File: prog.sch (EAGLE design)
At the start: 49 parts, among them IC2 LD398533RM, IC3 74AHCT1G04DBV, Q1 220mA/50V/3.5Ω, T1 SS8050-G, T2 SS8050-G, U1 SN74AHC125PWR, U2 FT2232HL-REEL

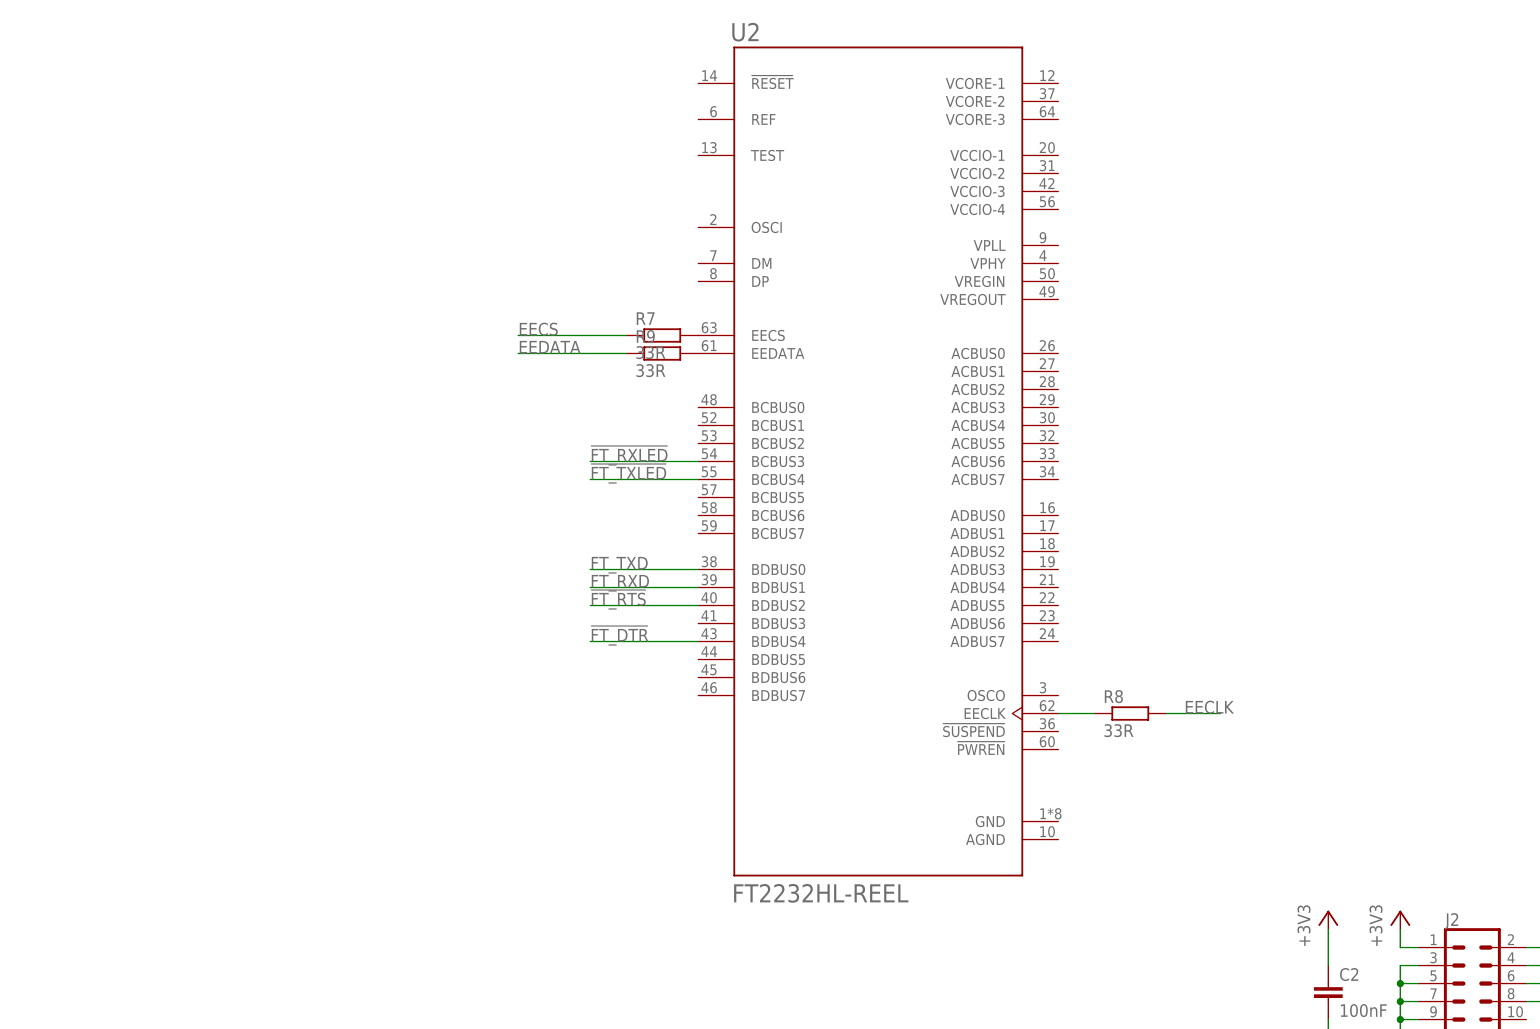
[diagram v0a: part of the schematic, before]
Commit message: work on programmer board
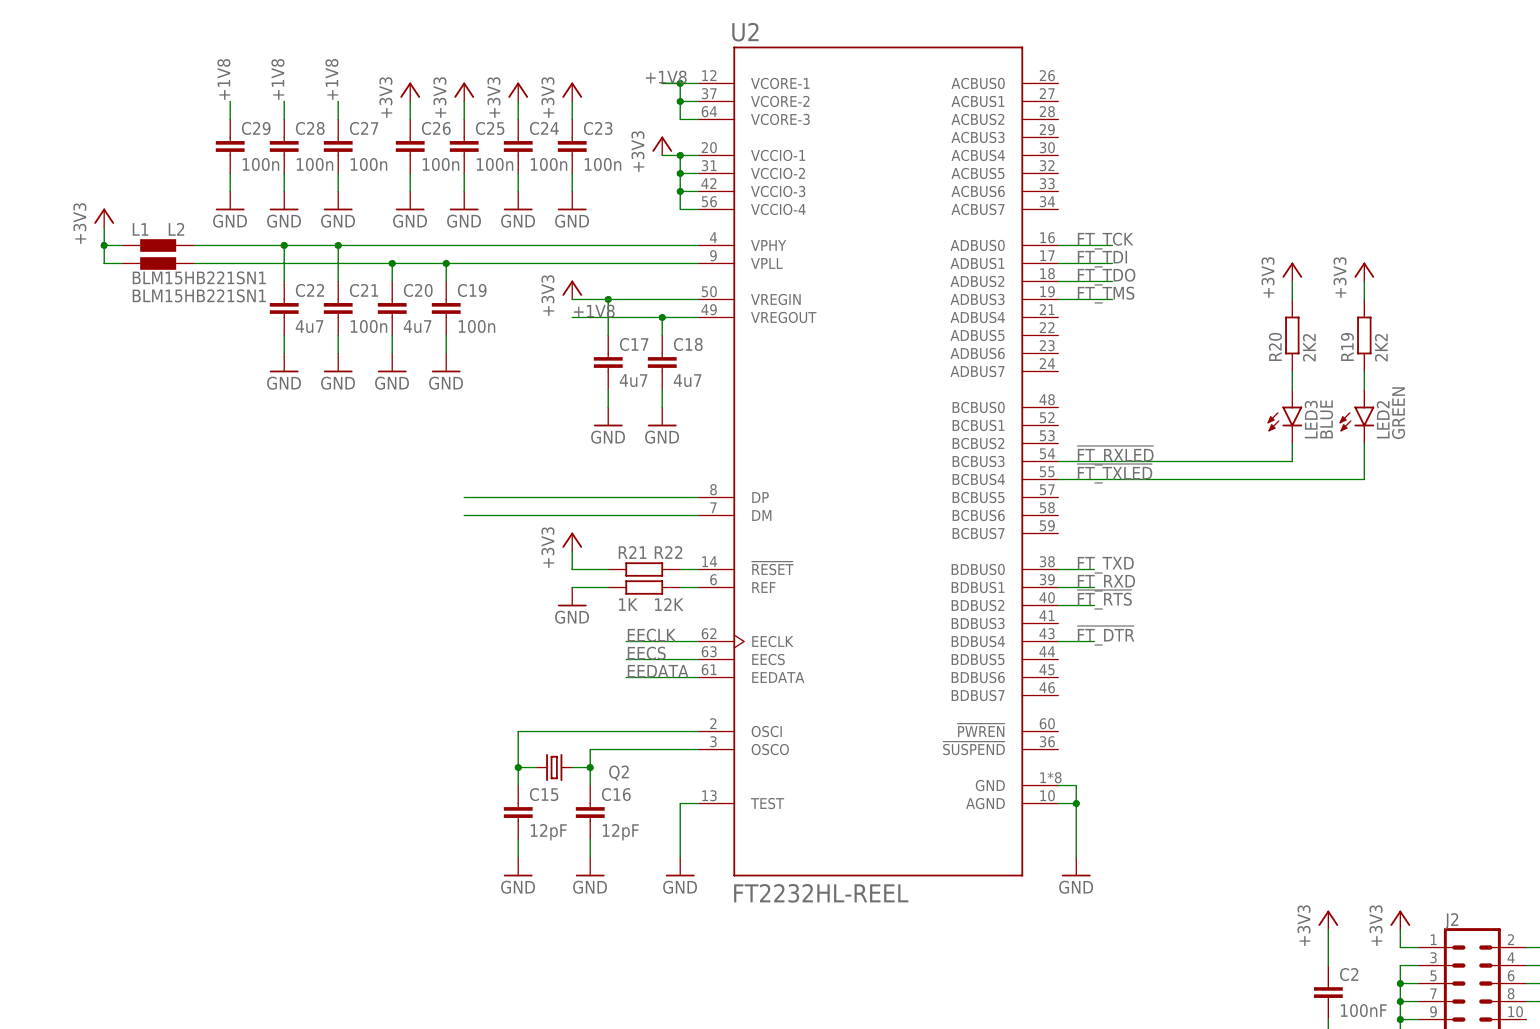
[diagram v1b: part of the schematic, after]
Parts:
- removed R7, R8, R9: 33R, resistor:R-EU_R0805
- added C15, C16: 12pF, resistor:C-EUC0805
- added C17, C18, C20, C22: 4u7, resistor:C-EUC0805
- added C19, C21, C23, C24, C25, C26, C27, C28, C29: 100n, resistor:C-EUC0805
- added L1, L2: BLM15HB221SN1, inductors:BLM15HB221SN1
- added LED2: GREEN, led:LEDCHIPLED_0805
- added LED3: BLUE, led:LEDCHIPLED_0805
- added Q2: (no value), crystal:CRYSTALHC49UP
- added R19, R20: 2K2, resistor:R-EU_R0805
- added R21: 12K, resistor:R-EU_R0805
- added R22: 1K, resistor:R-EU_R0805
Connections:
- removed net N$3: R7.2, U2.EECS
- removed net N$5: R9.2, U2.EEDATA
- removed net N$6: R8.2, U2.EECLK
- new net +1V8: C18.1, C27.1, C28.1, C29.1, U2.VCORE-1, U2.VCORE-2, U2.VCORE-3, U2.VREGOUT
- new net N$11: LED3.A, R20.1
- new net N$12: LED2.A, R19.1
- new net N$13: C15.1, Q2.1, U2.OSCI
- new net N$14: C16.1, Q2.2, U2.OSCO
- new net N$15: R22.2, U2.!RESET
- new net N$16: R21.2, U2.REF
- new net N$17: U2.DP
- new net N$18: U2.DM
- new net N$19: C19.1, C20.1, L2.2, U2.VPLL
- new net N$20: C21.1, C22.1, L1.2, U2.VPHY
- net !FT_RXLED: now also LED3.C
- net !FT_TXLED: now also LED2.C
- net +3V3: now also C17.1, C23.1, C24.1, C25.1, C26.1, L1.1, L2.1, R19.2, R20.2, R22.1, U2.VCCIO-1, U2.VCCIO-2, U2.VCCIO-3, U2.VCCIO-4, U2.VREGIN
- net EECLK: now also U2.EECLK; no longer R8.1
- net EECS: now also U2.EECS; no longer R7.1
- net EEDATA: now also U2.EEDATA; no longer R9.1
- net FT_TCK: now also U2.ADBUS0
- net FT_TDI: now also U2.ADBUS1
- net FT_TDO: now also U2.ADBUS2
- net FT_TMS: now also U2.ADBUS3
- net GND: now also C15.2, C16.2, C17.2, C18.2, C19.2, C20.2, C21.2, C22.2, C23.2, C24.2, C25.2, C26.2, C27.2, C28.2, C29.2, R21.1, U2.AGND, U2.GND, U2.TEST
